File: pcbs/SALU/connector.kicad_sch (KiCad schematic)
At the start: 13 parts, among them J201 Conn_02x20_Odd_Even, U201 74HC245, U202 74HC245

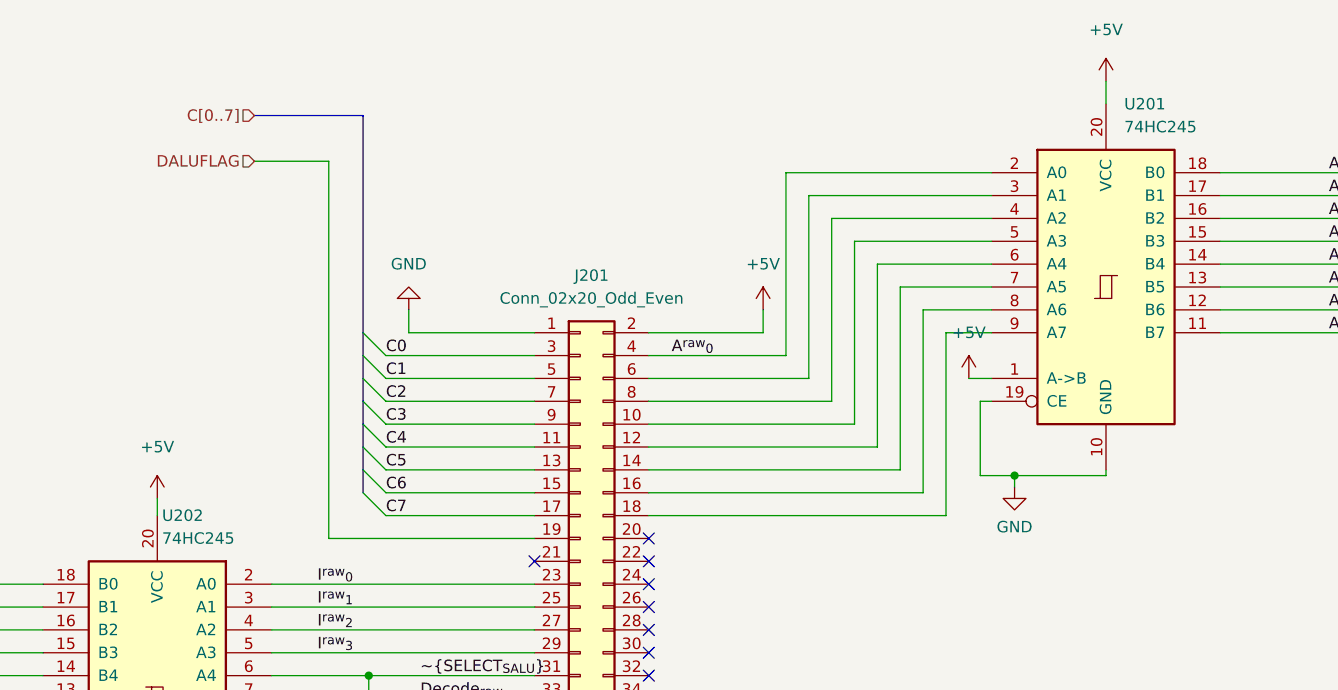
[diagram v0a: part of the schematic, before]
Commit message: Some more functions
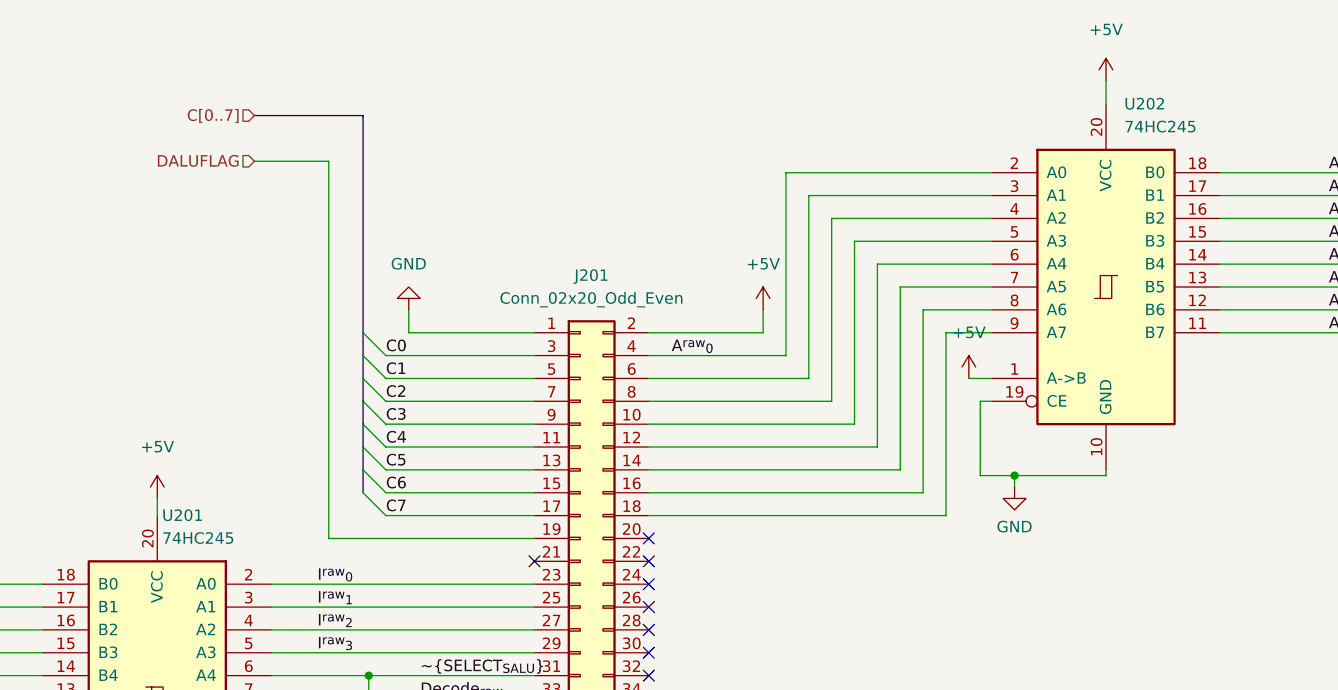
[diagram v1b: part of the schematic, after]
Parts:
- renumbered U202 to U201, U201 to U202
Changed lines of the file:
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@@
   (symbol (lib_id "power:GND") (at 60.325 113.665 0) (unit 1)
     (in_bom yes) (on_board yes) (fields_autoplaced)
-    (property "Reference" "#PWR0210" (id 0) (at 60.325 120.015 0)
+    (property "Reference" "#PWR0202" (id 0) (at 60.325 120.015 0)
       (effects (font (size 1.27 1.27)) hide)
     )
@@
   (symbol (lib_id "power:+5V") (at 60.325 70.485 0) (unit 1)
     (in_bom yes) (on_board yes) (fields_autoplaced)
-    (property "Reference" "#PWR0206" (id 0) (at 60.325 74.295 0)
+    (property "Reference" "#PWR0201" (id 0) (at 60.325 74.295 0)
       (effects (font (size 1.27 1.27)) hide)
     )
@@
   (symbol (lib_id "power:GND") (at 88.265 102.87 0) (unit 1)
     (in_bom yes) (on_board yes) (fields_autoplaced)
-    (property "Reference" "#PWR0208" (id 0) (at 88.265 109.22 0)
+    (property "Reference" "#PWR0205" (id 0) (at 88.265 109.22 0)
       (effects (font (size 1.27 1.27)) hide)
     )
@@
   (symbol (lib_id "power:+5V") (at 127.635 102.87 180) (unit 1)
     (in_bom yes) (on_board yes) (fields_autoplaced)
-    (property "Reference" "#PWR0209" (id 0) (at 127.635 99.06 0)
+    (property "Reference" "#PWR0210" (id 0) (at 127.635 99.06 0)
       (effects (font (size 1.27 1.27)) hide)
     )
@@
   (symbol (lib_id "power:+5V") (at 109.22 154.94 270) (unit 1)
     (in_bom yes) (on_board yes) (fields_autoplaced)
-    (property "Reference" "#PWR0214" (id 0) (at 105.41 154.94 0)
+    (property "Reference" "#PWR0206" (id 0) (at 105.41 154.94 0)
       (effects (font (size 1.27 1.27)) hide)
     )
@@
   (symbol (lib_id "power:GND") (at 88.265 49.53 180) (unit 1)
     (in_bom yes) (on_board yes) (fields_autoplaced)
-    (property "Reference" "#PWR0202" (id 0) (at 88.265 43.18 0)
+    (property "Reference" "#PWR0204" (id 0) (at 88.265 43.18 0)
       (effects (font (size 1.27 1.27)) hide)
     )
@@
   (symbol (lib_id "power:+5V") (at 196.85 130.81 0) (unit 1)
     (in_bom yes) (on_board yes) (fields_autoplaced)
-    (property "Reference" "#PWR0212" (id 0) (at 196.85 134.62 0)
+    (property "Reference" "#PWR0214" (id 0) (at 196.85 134.62 0)
       (effects (font (size 1.27 1.27)) hide)
     )
@@
   (symbol (lib_id "power:GND") (at 110.49 179.07 90) (mirror x) (unit 1)
     (in_bom yes) (on_board yes) (fields_autoplaced)
-    (property "Reference" "#PWR0215" (id 0) (at 116.84 179.07 0)
+    (property "Reference" "#PWR0208" (id 0) (at 116.84 179.07 0)
       (effects (font (size 1.27 1.27)) hide)
     )
@@
   (symbol (lib_id "power:GND") (at 155.575 69.215 0) (unit 1)
     (in_bom yes) (on_board yes) (fields_autoplaced)
-    (property "Reference" "#PWR0205" (id 0) (at 155.575 75.565 0)
+    (property "Reference" "#PWR0212" (id 0) (at 155.575 75.565 0)
       (effects (font (size 1.27 1.27)) hide)
     )
@@
   (symbol (lib_id "power:GND") (at 197.485 142.875 0) (unit 1)
     (in_bom yes) (on_board yes) (fields_autoplaced)
-    (property "Reference" "#PWR0213" (id 0) (at 197.485 149.225 0)
+    (property "Reference" "#PWR0215" (id 0) (at 197.485 149.225 0)
       (effects (font (size 1.27 1.27)) hide)
     )
@@
   (symbol (lib_id "74xx:74HC245") (at 60.325 92.71 0) (mirror y) (unit 1)
     (in_bom yes) (on_board yes) (fields_autoplaced)
-    (property "Reference" "U202" (id 0) (at 60.8456 72.39 0)
+    (property "Reference" "U201" (id 0) (at 60.8456 72.39 0)
       (effects (font (size 1.27 1.27)) (justify right))
     )
@@
   (symbol (lib_id "74xx:74HC245") (at 165.735 46.99 0) (unit 1)
     (in_bom yes) (on_board yes) (fields_autoplaced)
-    (property "Reference" "U201" (id 0) (at 167.7544 26.67 0)
+    (property "Reference" "U202" (id 0) (at 167.7544 26.67 0)
       (effects (font (size 1.27 1.27)) (justify left))
     )
@@
   (symbol (lib_id "power:+5V") (at 150.495 57.15 0) (unit 1)
     (in_bom yes) (on_board yes) (fields_autoplaced)
-    (property "Reference" "#PWR0204" (id 0) (at 150.495 60.96 0)
+    (property "Reference" "#PWR0211" (id 0) (at 150.495 60.96 0)
       (effects (font (size 1.27 1.27)) hide)
     )
@@
   (symbol (lib_id "power:+5V") (at 76.2 102.87 270) (unit 1)
     (in_bom yes) (on_board yes) (fields_autoplaced)
-    (property "Reference" "#PWR0207" (id 0) (at 72.39 102.87 0)
+    (property "Reference" "#PWR0203" (id 0) (at 72.39 102.87 0)
       (effects (font (size 1.27 1.27)) hide)
     )
@@
   (symbol (lib_id "power:+5V") (at 127.635 49.53 0) (unit 1)
     (in_bom yes) (on_board yes) (fields_autoplaced)
-    (property "Reference" "#PWR0203" (id 0) (at 127.635 53.34 0)
+    (property "Reference" "#PWR0209" (id 0) (at 127.635 53.34 0)
       (effects (font (size 1.27 1.27)) hide)
     )
@@
   (symbol (lib_id "power:GND") (at 110.49 130.175 90) (mirror x) (unit 1)
     (in_bom yes) (on_board yes) (fields_autoplaced)
-    (property "Reference" "#PWR0211" (id 0) (at 116.84 130.175 0)
+    (property "Reference" "#PWR0207" (id 0) (at 116.84 130.175 0)
       (effects (font (size 1.27 1.27)) hide)
     )
@@
   (symbol (lib_id "power:+5V") (at 165.735 24.13 0) (unit 1)
     (in_bom yes) (on_board yes) (fields_autoplaced)
-    (property "Reference" "#PWR0201" (id 0) (at 165.735 27.94 0)
-      (effects (font (size 1.27 1.27)) hide)
-    )
+    (property "Reference" "#PWR0213" (id 0) (at 165.735 27.94 0)
+      (effects (font (size 1.27 1.27)) hide)
+    )
